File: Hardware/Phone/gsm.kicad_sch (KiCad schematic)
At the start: 28 parts

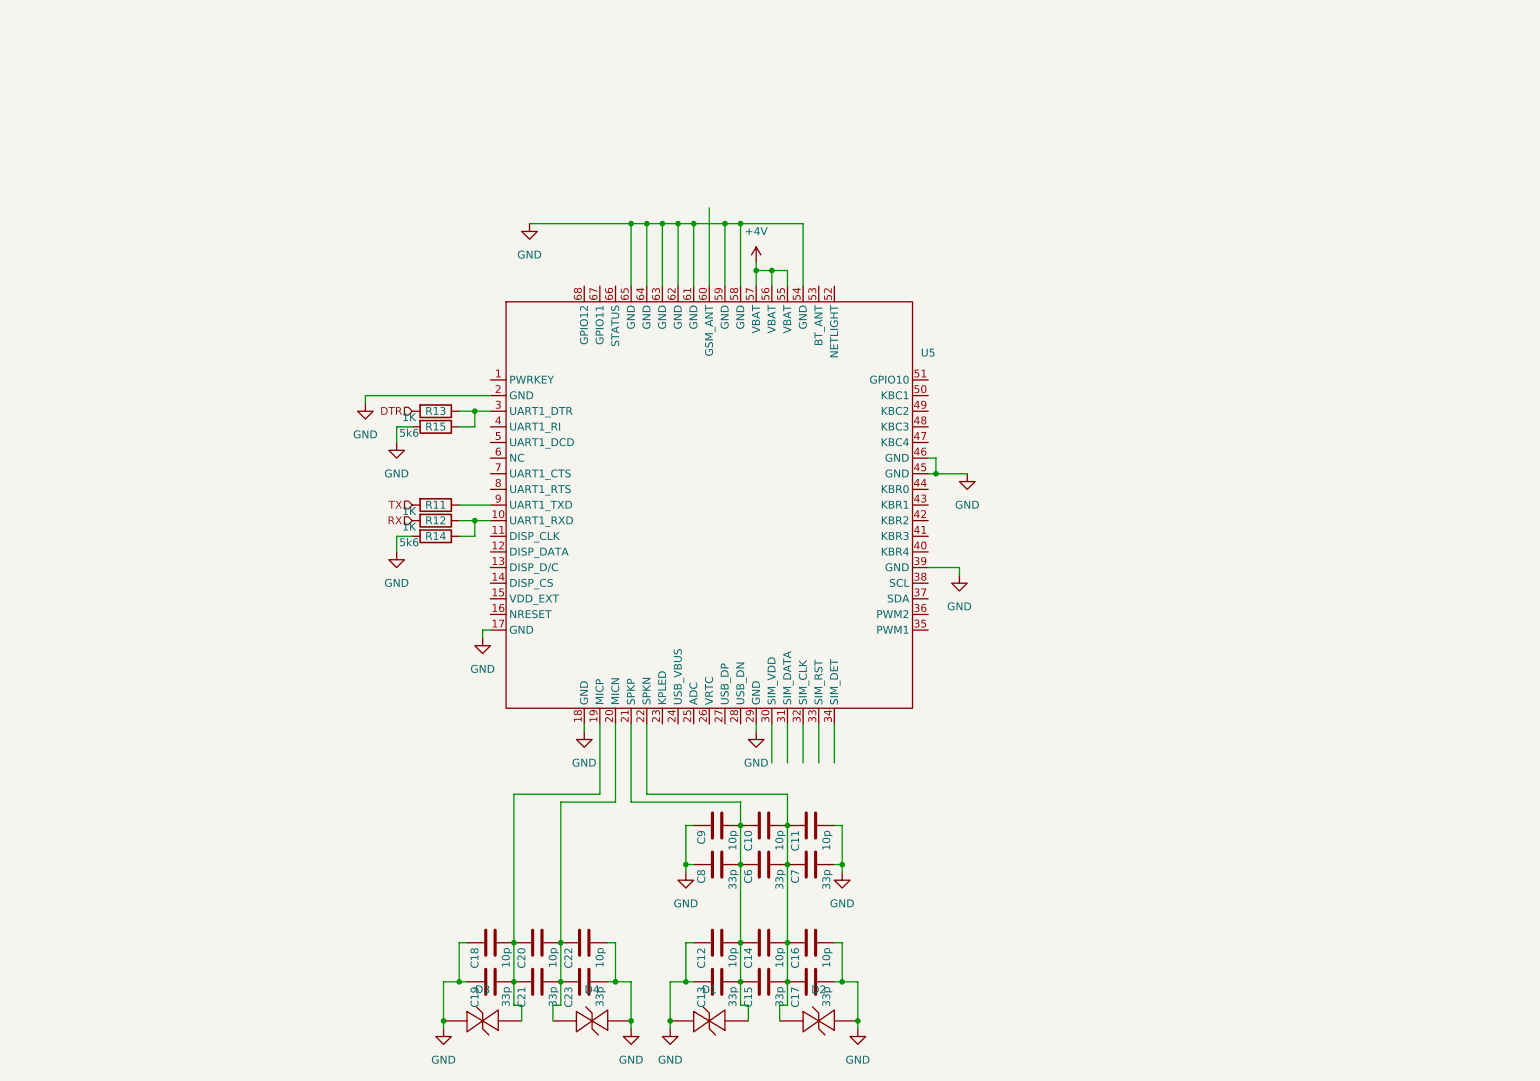
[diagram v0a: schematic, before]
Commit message: e ink is done
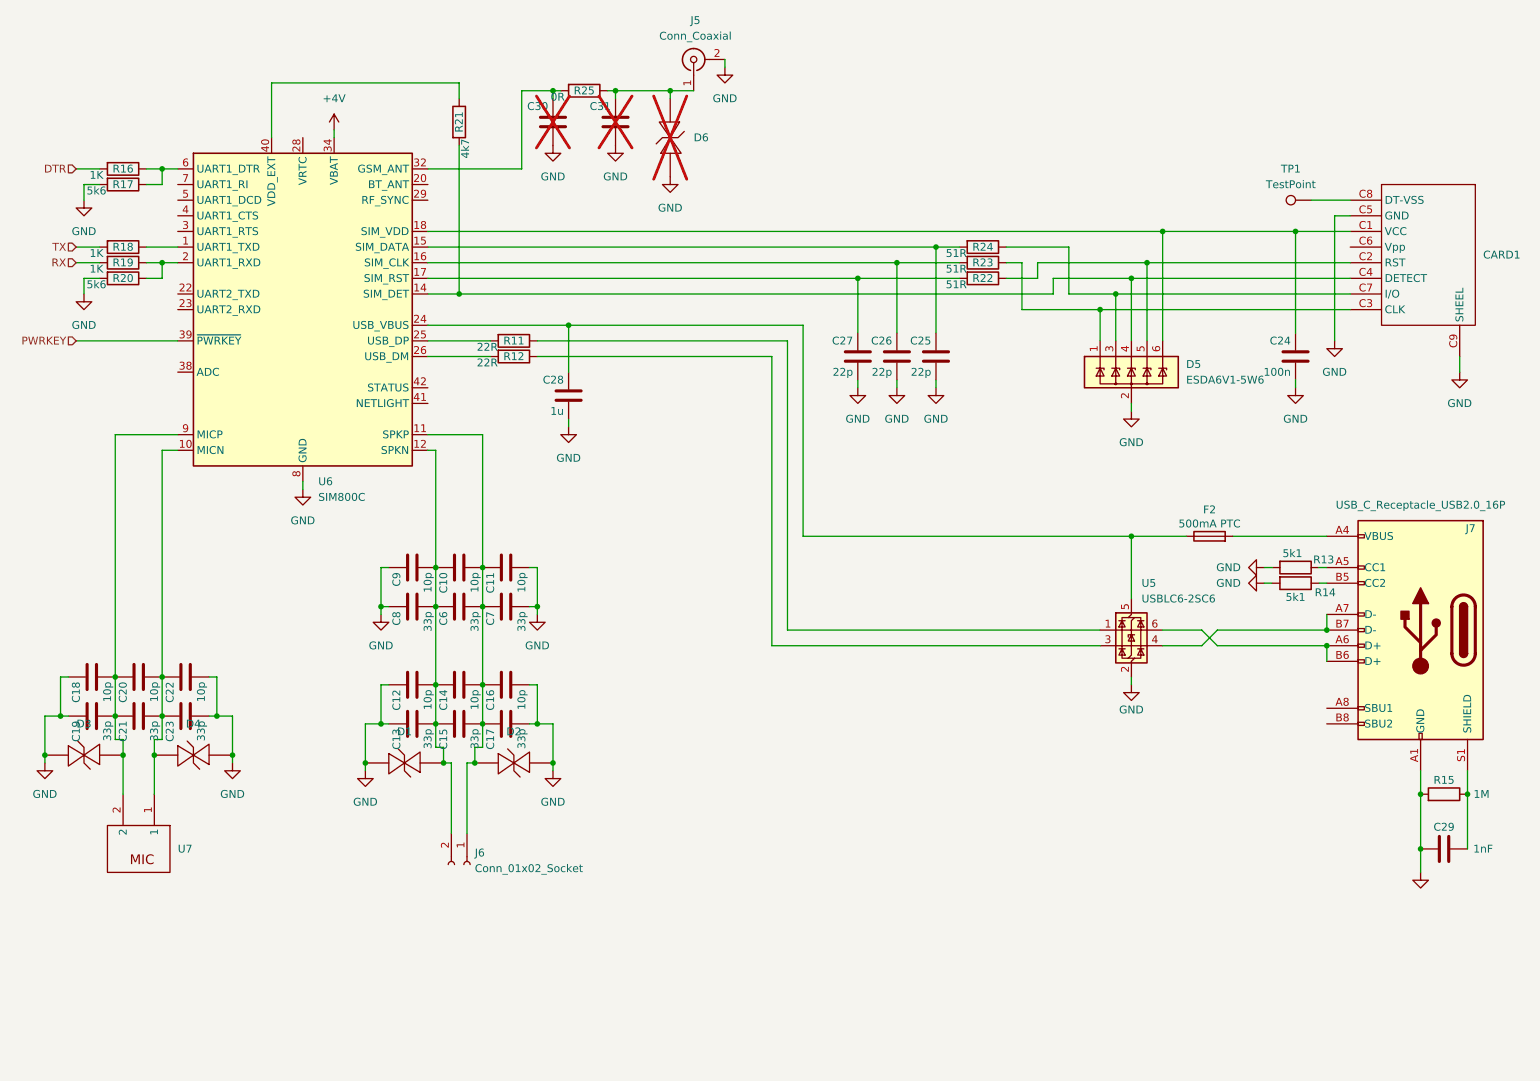
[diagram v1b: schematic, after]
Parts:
- removed U5: ~, Felix_GSM:GSMM-SMD_SIM800A32M, symbol Felix_GSM:SIM800A 32m
- added C24: 100n, Capacitor_SMD:C_0603_1608Metric, symbol Device:C
- added C25, C26, C27: 22p, Capacitor_SMD:C_0603_1608Metric, symbol Device:C
- added C28: 1u, Capacitor_SMD:C_0603_1608Metric, symbol Device:C
- added C29: 1nF, Capacitor_SMD:C_1206_3216Metric, symbol Device:C
- added C30, C31: ~, Capacitor_SMD:C_0603_1608Metric, symbol Device:C
- added CARD1: ~, Felix_GSM:SIM-SMD_503960-0696, symbol Felix_GSM:503960-0696
- added D5: ESDA6V1-5W6, Package_TO_SOT_SMD:SOT-363_SC-70-6, symbol Power_Protection:ESDA6V1-5SC6
- added D6: ~, Felix:SOD-882_L1.0-W0.6-BI, symbol Felix:H5VL10B
- added F2: 500mA PTC, Fuse:Fuse_1206_3216Metric_Pad1.42x1.75mm_HandSolder, symbol Device:Fuse
- added J5: Conn_Coaxial, Connector_Coaxial:U.FL_Hirose_U.FL-R-SMT-1_Vertical, symbol Connector:Conn_Coaxial
- added J6: Conn_01x02_Socket, Connector_PinHeader_2.54mm:PinHeader_1x02_P2.54mm_Vertical, symbol Connector:Conn_01x02_Socket
- added J7: USB_C_Receptacle_USB2.0_16P, Connector_USB:USB_C_Receptacle_HRO_TYPE-C-31-M-12, symbol Connector:USB_C_Receptacle_USB2.0_16P
- added R16, R18, R19: 1K, Resistor_SMD:R_0603_1608Metric, symbol Device:R
- added R17, R20: 5k6, Resistor_SMD:R_0603_1608Metric, symbol Device:R
- added R21: 4k7, Resistor_SMD:R_0603_1608Metric, symbol Device:R
- added R22, R23, R24: 51R, Resistor_SMD:R_0603_1608Metric, symbol Device:R
- added R25: 0R, Resistor_SMD:R_0603_1608Metric, symbol Device:R
- added TP1: TestPoint, TestPoint:TestPoint_Pad_D1.0mm, symbol Connector:TestPoint
- added U5: USBLC6-2SC6, Package_TO_SOT_SMD:SOT-23-6, symbol Power_Protection:USBLC6-2SC6
- added U6: SIM800C, RF_GSM:SIMCom_SIM800C, symbol RF_GSM:SIM800C
- added U7: ~, Felix:MIC-TH_BD4.0-P1.40_KEEG1542PBL-A, symbol Felix:KEEG1542PBL-A
- R11, R12: value 1K -> 22R
- R13: value 1K -> 5k1; footprint Resistor_SMD:R_0603_1608Metric -> Resistor_SMD:R_1206_3216Metric
- R14: value 5k6 -> 5k1; footprint Resistor_SMD:R_0603_1608Metric -> Resistor_SMD:R_1206_3216Metric
- R15: value 5k6 -> 1M; footprint Resistor_SMD:R_0603_1608Metric -> Resistor_SMD:R_1206_3216Metric
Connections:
- net +4V: now also U6.34 (VBAT), U6.35 (VBAT)
- net DTR: now also R16.2; no longer R13.2
- net GND: now also R13.2, C24.1, C25.1, C26.1, C27.1, C28.1, C29.2, C30.1, C31.1, CARD1.C5 (GND), CARD1.C9 (SHEEL), D5.2 (GND), D6.2 (A), J5.2 (Ext), J7.A1 (GND), J7.A12 (GND), J7.B1 (GND), J7.B12 (GND), R17.2, R20.2, U5.2 (GND), U6.13 (GND), U6.19 (GND), U6.21 (GND), U6.27 (GND), U6.30 (GND), U6.31 (GND), U6.33 (GND), U6.36 (GND), U6.37 (GND), U6.8 (GND)
- net RX: now also R19.2; no longer R12.2
- net TX: now also R18.2; no longer R11.2
- net at C20.1, C21.1, C22.2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: now also U6.10 (MICN), U7.1
- net at C18.1, C19.1, C20.2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: now also U6.9 (MICP), U7.2
- net at R13.1: now also J7.A5 (CC1); no longer R15.1
- net at C10.1, C11.2, C14.1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: now also J6.1 (Pin_1), U6.11 (SPKP)
- net at C10.2, C12.1, C13.1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: now also J6.2 (Pin_2), U6.12 (SPKN)
- net at R12.1: now also U5.3 (I/O2); no longer R14.1
- net at R11.1: now also U5.1 (I/O1)
- new net: R19.1, R20.1, U6.2 (UART1_RXD)
- new net: C28.2, F2.1, U5.5 (VBUS), U6.24 (USB_VBUS)
- new net: F2.2, J7.A4 (VBUS), J7.A9 (VBUS), J7.B4 (VBUS), J7.B9 (VBUS)
- new net: CARD1.C3 (CLK), D5.1 (IO1), R23.1
- new net: CARD1.C7 (I/O), D5.3 (IO2), R24.1
- new net: CARD1.C4 (DETECT), D5.4 (IO3), R21.2, U6.14 (SIM_DET)
- new net: CARD1.C2 (RST), D5.5 (IO4), R22.1
- new net: C24.2, CARD1.C1 (VCC), D5.6 (IO5), U6.18 (SIM_VDD)
- new net: C26.2, R23.2, U6.16 (SIM_CLK)
- new net: CARD1.C8 (DT-VSS), TP1.1
- new net: R12.2, U6.26 (USB_DM)
- new net: C31.2, D6.1 (C), J5.1 (In), R25.1
- new net: R16.1, R17.1, U6.6 (UART1_DTR)
- new net: C30.2, R25.2, U6.32 (GSM_ANT)
- new net: C27.2, R22.2, U6.17 (SIM_RST)
- new net: C25.2, R24.2, U6.15 (SIM_DATA)
- new net: J7.A7 (D-), J7.B7 (D-), U5.4 (I/O2)
- new net: J7.A6 (D+), J7.B6 (D+), U5.6 (I/O1)
- new net: R11.2, U6.25 (USB_DP)
- new net: R18.1, U6.1 (UART1_TXD)
- new net: J7.B5 (CC2), R14.1
- new net: C29.1, J7.S1 (SHIELD), R15.1
- new net: R21.1, U6.40 (VDD_EXT)
- new net PWRKEY: U6.39 (~{PWRKEY})
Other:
- moved on the sheet: C10, C11, C12, C13, C14, C15, C16, C17, C18, C19, C20, C21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
